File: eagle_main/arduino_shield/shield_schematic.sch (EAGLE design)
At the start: 17 parts, among them IC1 74LS595D, J1 ARDUINO_R3_SHIELD

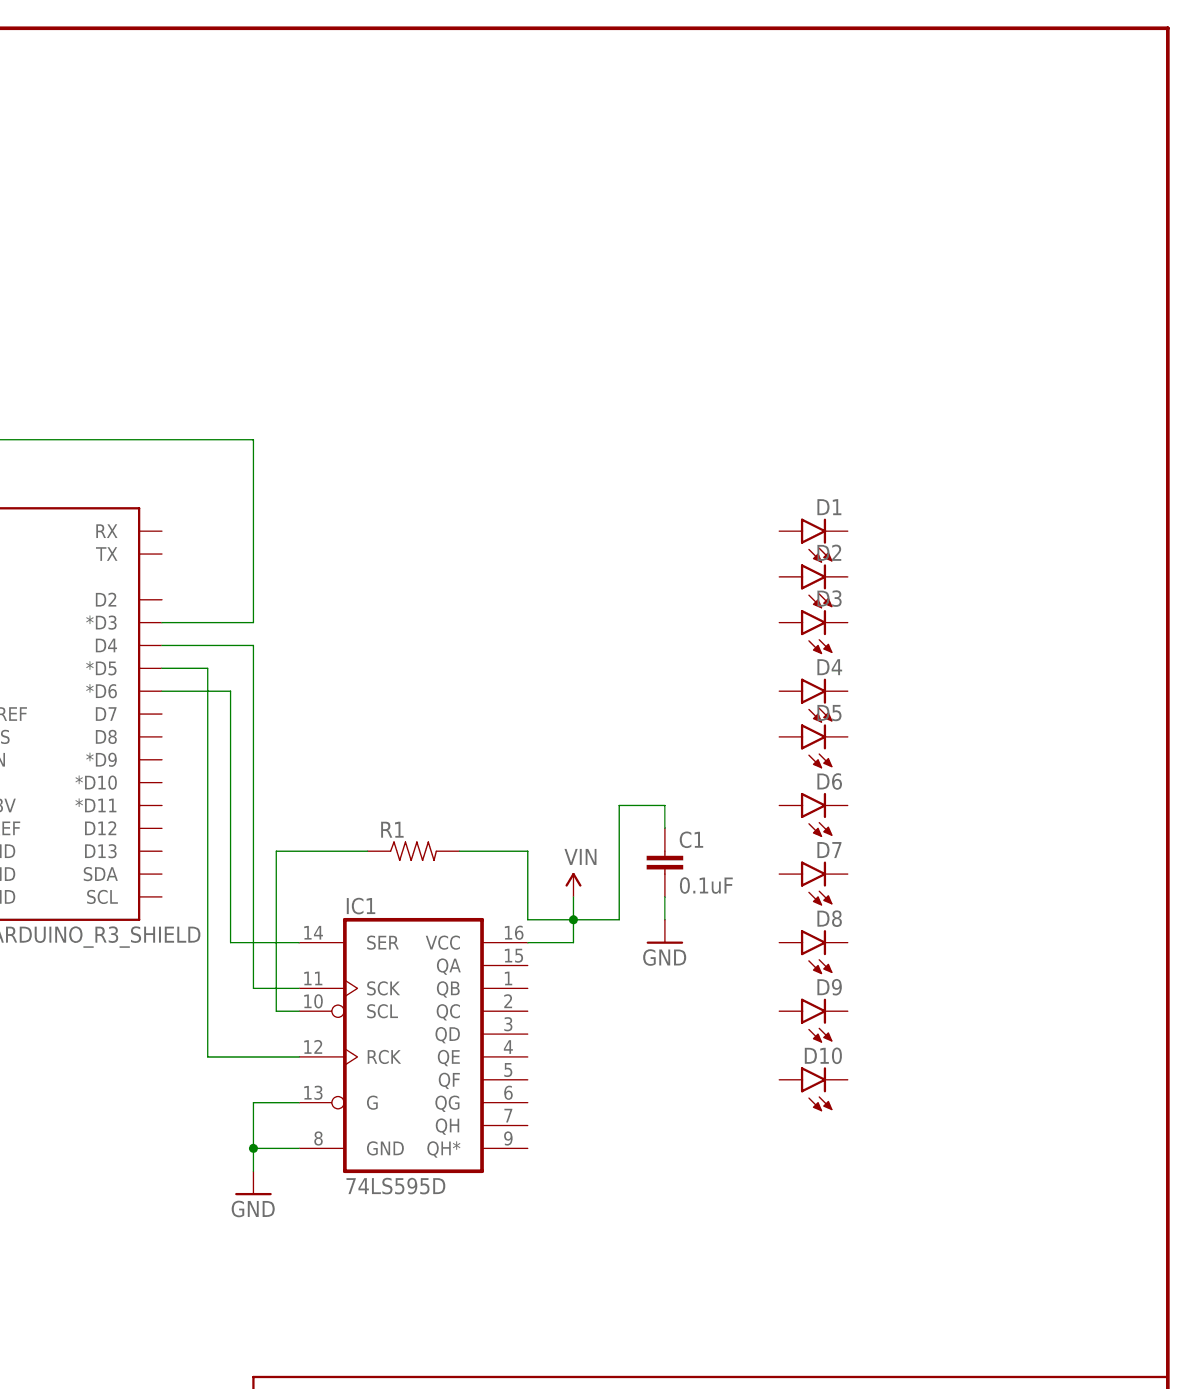
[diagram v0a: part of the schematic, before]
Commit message: Updated parts for November 4th
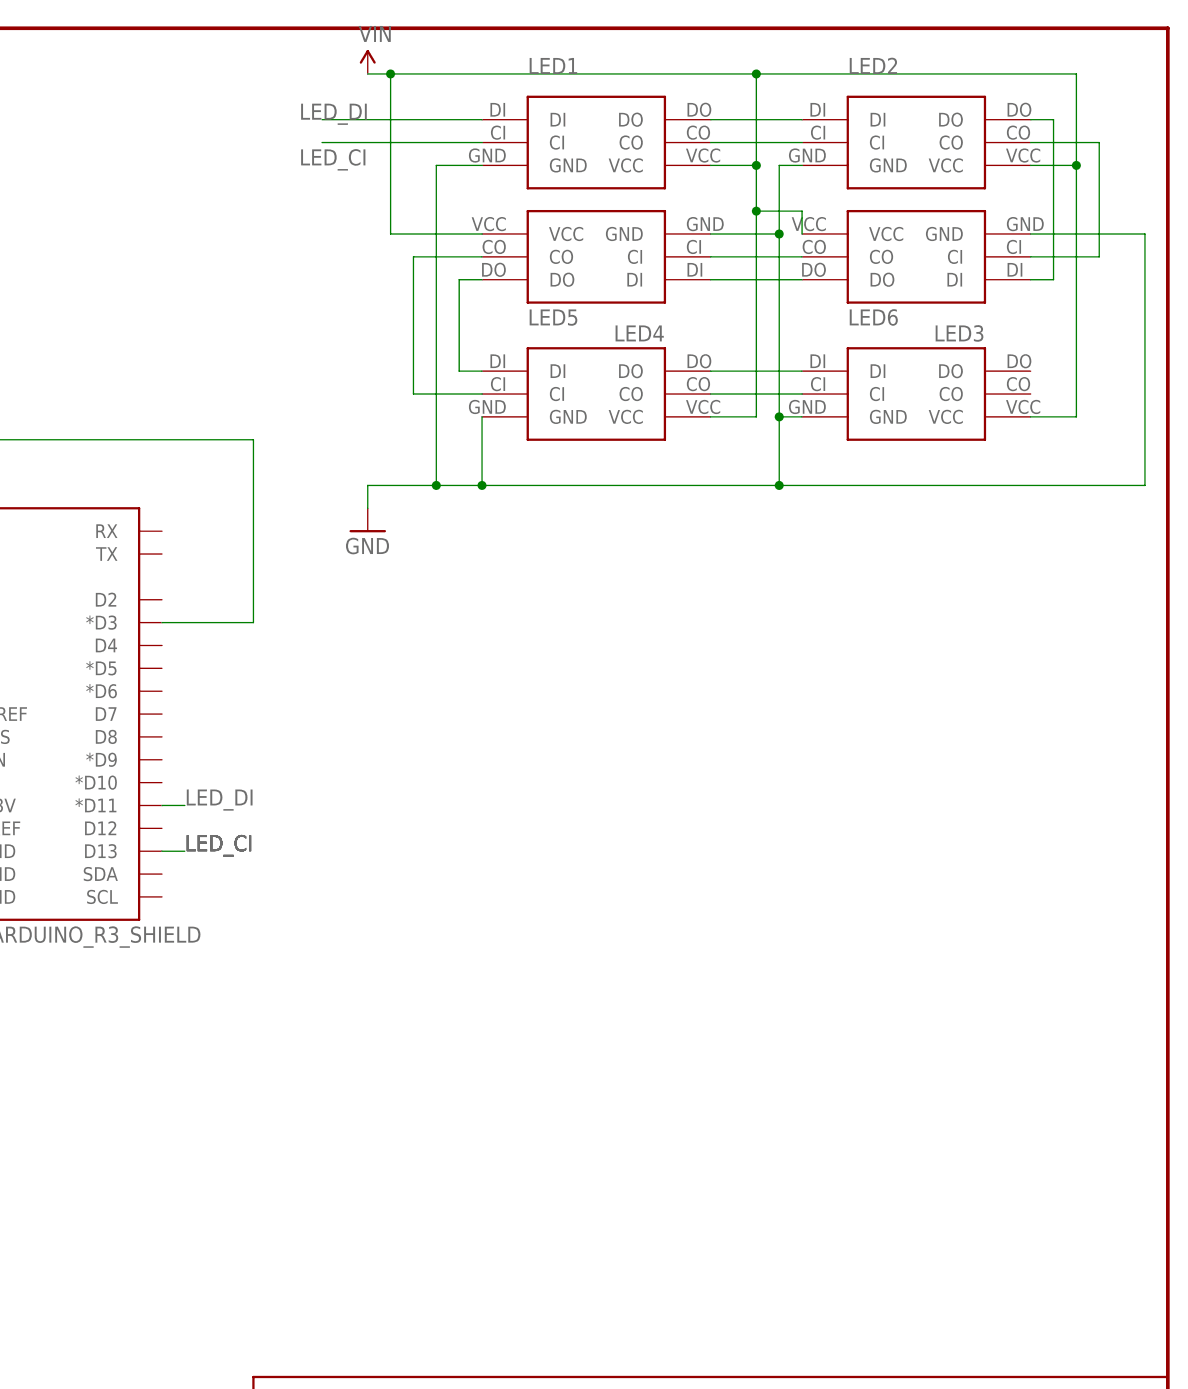
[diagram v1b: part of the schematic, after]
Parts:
- removed C1: 0.1uF, SparkFun-Capacitors:CAP0603-CAP
- removed D1, D10, D2, D3, D4, D5, D6, D7, D8, D9: (no value), SparkFun-LED:LED5MM
- removed IC1: 74LS595D, SparkFun-DigitalIC:74LS595D
- removed R1: (no value), SparkFun-Resistors:RESISTOR0603
- added LED1, LED2, LED3, LED4, LED5, LED6: APA102SMD, Arduino_Shield:APA102SMD
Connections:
- removed net N$4: IC1.SCK, J1.D4
- removed net N$5: IC1.RCK, J1.*D5
- removed net N$6: IC1.SCL, R1.1
- removed net N$8: IC1.SER, J1.*D6
- new net LED_CI: J1.D13, LED1.CI
- new net LED_DI: J1.*D11, LED1.DI
- new net N$14: LED1.DO, LED2.DI
- new net N$15: LED1.CO, LED2.CI
- new net N$16: LED2.DO, LED3.DI
- new net N$17: LED2.CO, LED3.CI
- new net N$18: LED3.CO, LED4.CI
- new net N$19: LED3.DO, LED4.DI
- new net N$20: LED4.CO, LED5.CI
- new net N$21: LED4.DO, LED5.DI
- new net N$22: LED5.DO, LED6.DI
- new net N$23: LED5.CO, LED6.CI
- net GND: now also LED1.GND, LED2.GND, LED3.GND, LED4.GND, LED5.GND, LED6.GND; no longer C1.2, IC1.G, IC1.GND
- net VIN: now also LED1.VCC, LED2.VCC, LED3.VCC, LED4.VCC, LED5.VCC, LED6.VCC; no longer C1.1, IC1.VCC, R1.2
